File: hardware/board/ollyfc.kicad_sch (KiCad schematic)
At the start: 48 parts, among them J1 Conn_01x06, J12 Conn_01x08, J13 Conn_01x04, J5 Conn_02x05_Odd_Even, Q2 MMBT3904, Q3 MMBT3904, SW2 SW_Push, SW3 SW_Push, SW4 MODE1, SW5 MODE1, U3 STM32F411RETx, U6 W25Q128JVS, X1 X322516MLB4SI

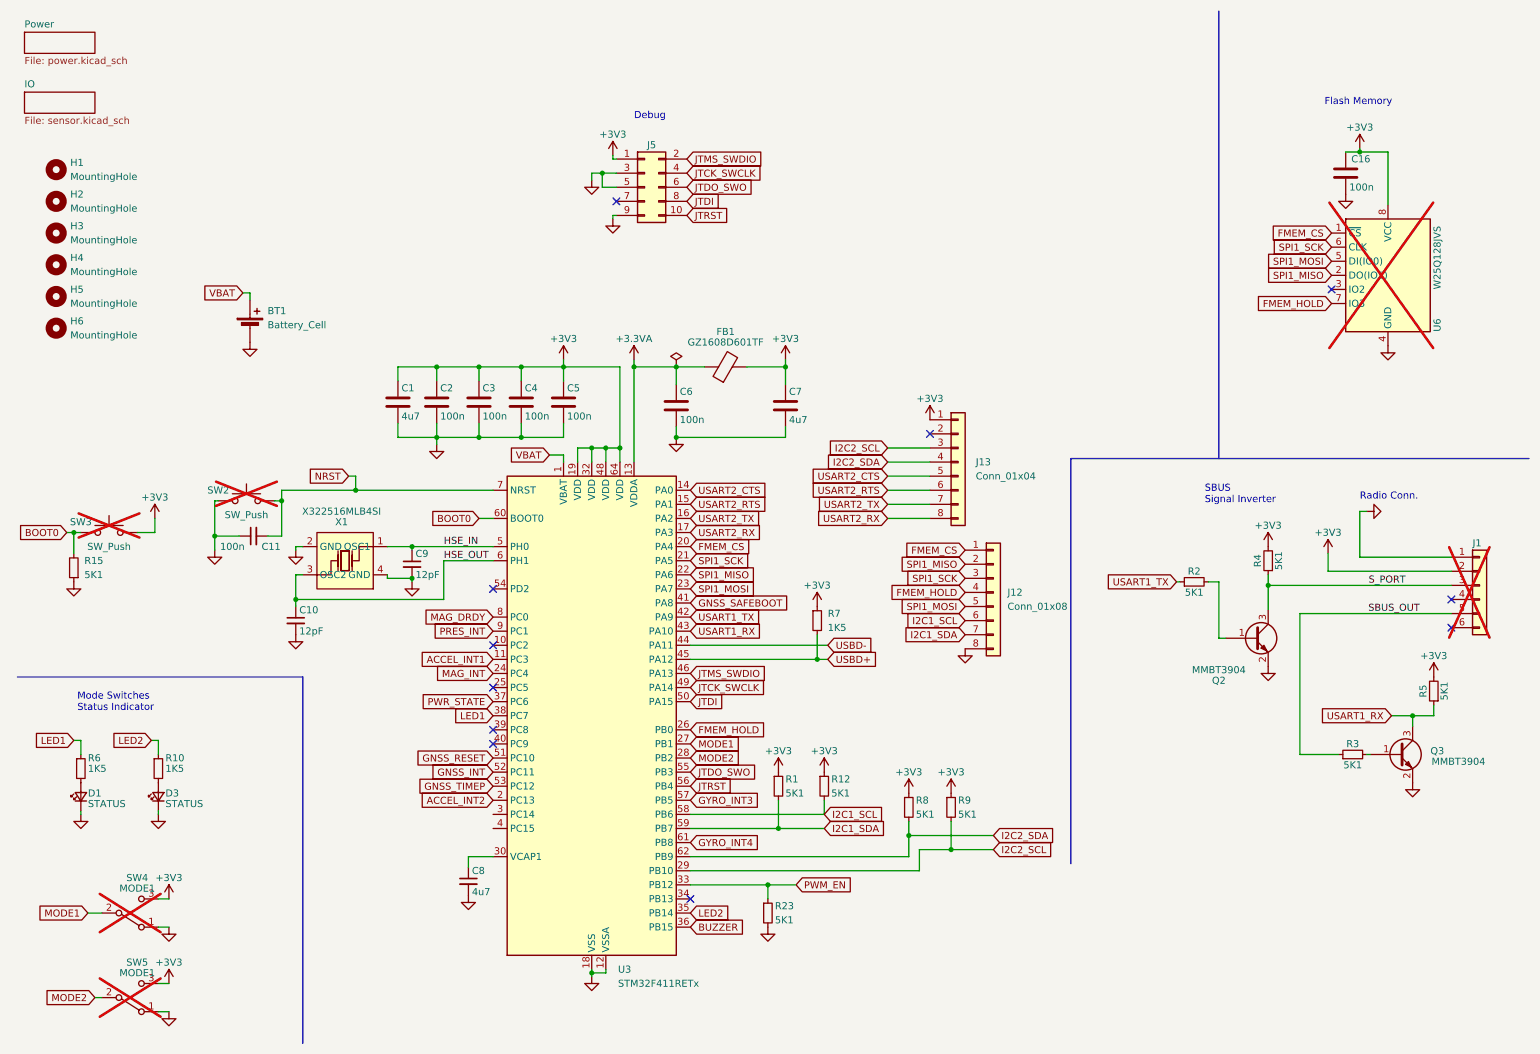
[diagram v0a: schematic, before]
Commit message: v2 files
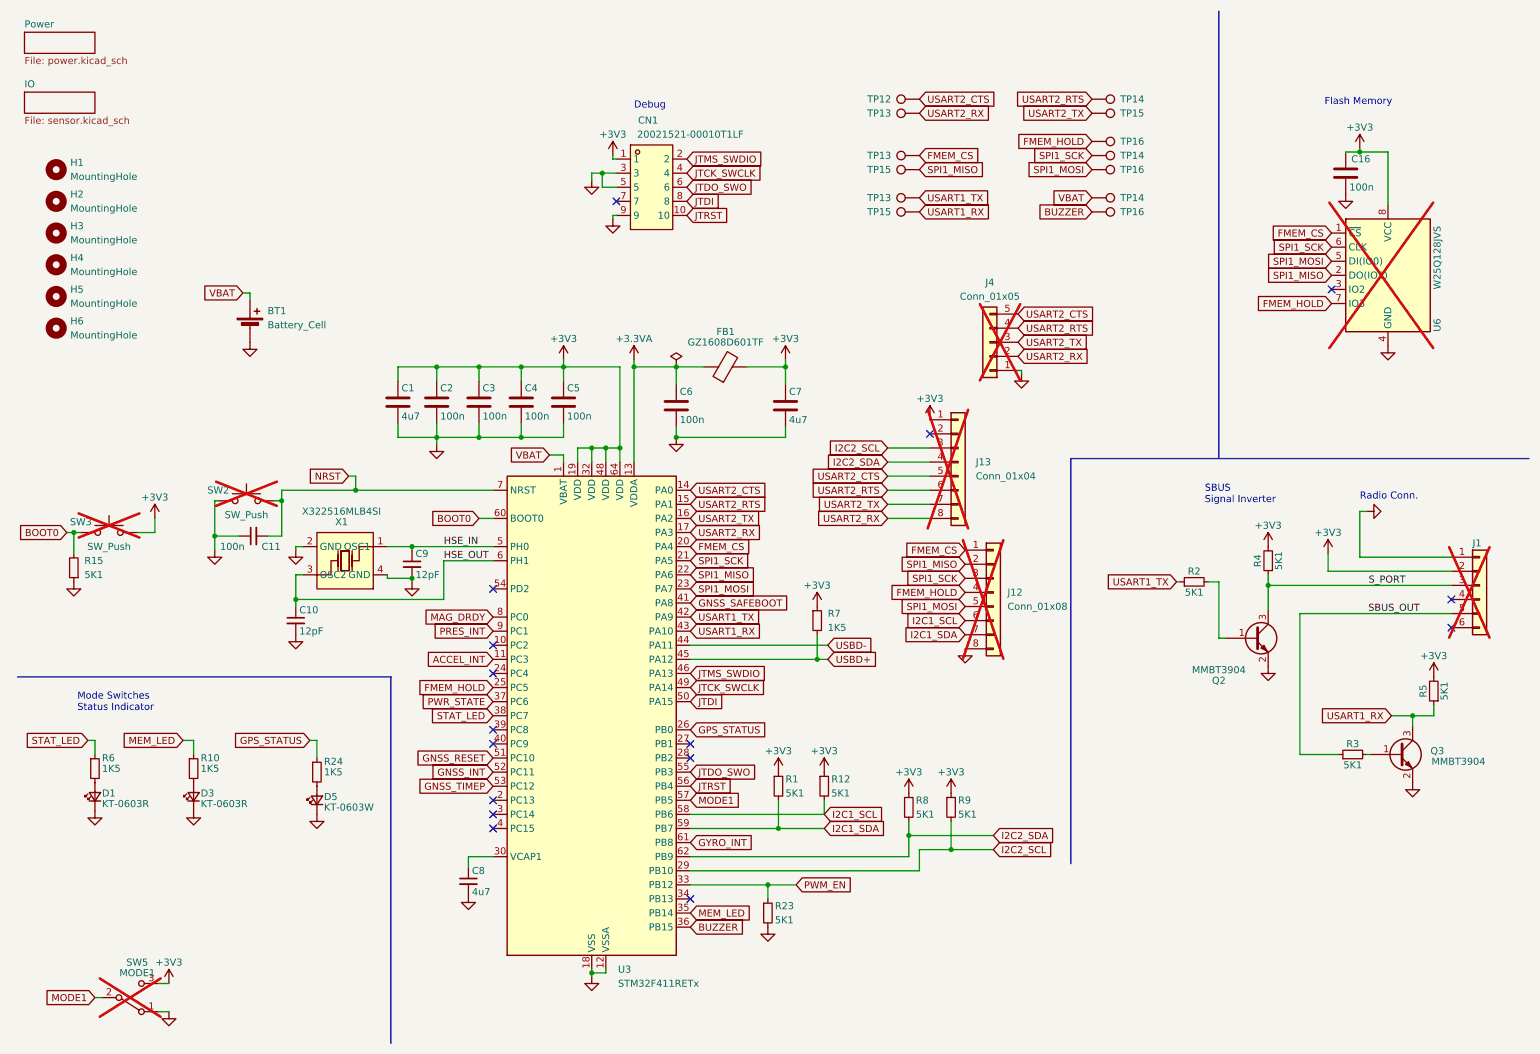
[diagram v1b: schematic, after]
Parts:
- removed J5: Conn_02x05_Odd_Even, Connector_PinHeader_1.27mm:PinHeader_2x05_P1.27mm_Vertical, symbol Connector_Generic:Conn_02x05_Odd_Even
- removed SW4: MODE1, Button_Switch_SMD:SW_SPDT_PCM12, symbol Switch:SW_SPDT
- added CN1: 20021521-00010T1LF, ofc_sym:IDC-SMD_10P-P1.27_X1270WVS-2X05B-6TV01, symbol ofc_sym:20021521-00010T1LF
- added D5: KT-0603W, ofc_sym:LED0603-R-RD_WHITE, symbol Device:LED_Small
- added J4: Conn_01x05, Connector_JST:JST_PH_B5B-PH-K_1x05_P2.00mm_Vertical, symbol Connector_Generic:Conn_01x05
- added R24: 1K5, Resistor_SMD:R_0402_1005Metric, symbol Device:R_Small
- added TP12, TP13 (x3), TP14 (x3), TP15 (x3), TP16 (x3): TestPoint, TestPoint:TestPoint_Pad_D1.5mm, symbol Connector:TestPoint
- BT1: now left out of the parts list
- C10, C9: footprint ofc_sym:C0402 -> Capacitor_SMD:C_0402_1005Metric; LCSC Part (none) -> C1547
- D1, D3: value STATUS -> KT-0603R; footprint LED_SMD:LED_0603_1608Metric -> ofc_sym:LED0603-RD
- J12, J13: now not fitted; now left out of the parts list
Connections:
- net GYRO_INT3 is gone; now on net MODE1: U3.57 (PB5)
- net +3V3: now also CN1.1
- net BUZZER: now also TP16.1
- net FMEM_CS: now also TP13.1
- net FMEM_HOLD: now also U3.25 (PC5), TP16.1; no longer U3.26 (PB0)
- net GND: now also CN1.3, CN1.5, CN1.9, D5.1 (K), J4.1 (Pin_1)
- net JTCK_SWCLK: now also CN1.4
- net JTDI: now also CN1.8
- net JTDO_SWO: now also CN1.6
- net JTMS_SWDIO: now also CN1.2
- net JTRST: now also CN1.10
- net MODE1: now also SW5.2 (B); no longer U3.27 (PB1)
- net SPI1_MISO: now also TP15.1
- net SPI1_MOSI: now also TP16.1
- net SPI1_SCK: now also TP14.1
- net USART1_RX: now also TP15.1
- net USART1_TX: now also TP13.1
- net USART2_CTS: now also J4.5 (Pin_5), TP12.1
- net USART2_RTS: now also J4.4 (Pin_4), TP14.1
- net USART2_RX: now also J4.2 (Pin_2), TP13.1
- net USART2_TX: now also J4.3 (Pin_3), TP15.1
- net VBAT: now also TP14.1
- net ACCEL_INT1 renamed ACCEL_INT
- net ACCEL_INT2: no longer names the net of U3.2 (PC13)
- net GYRO_INT4 renamed GYRO_INT
- net LED1 renamed STAT_LED
- net LED2 renamed MEM_LED
- net MAG_INT: no longer names the net of U3.24 (PC4)
- net MODE2: no longer names the net of U3.28 (PB2)
- net MODE2: no longer SW5.2 (B)
- new net: D5.2 (A), R24.2
- new net GPS_STATUS: R24.1, U3.26 (PB0)
- no-connect marks 11 -> 16
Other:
- moved on the sheet: R10, R6
